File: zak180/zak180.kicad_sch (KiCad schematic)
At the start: 1 part, among them X1 25.175 MHz

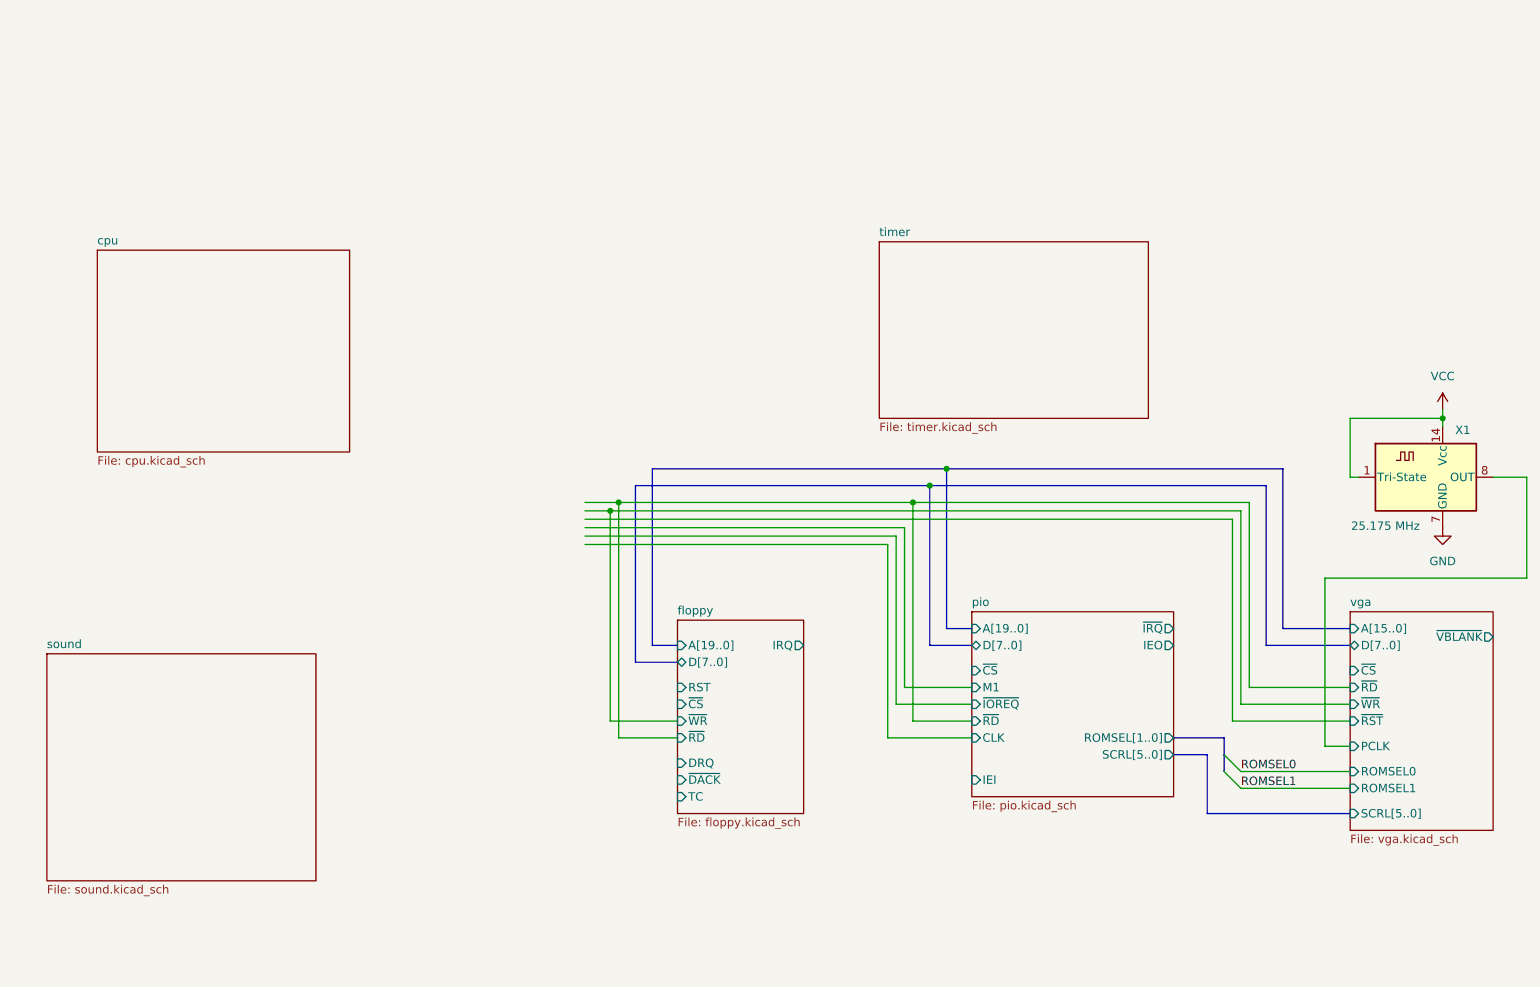
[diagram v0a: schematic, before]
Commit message: HW: Further work on schematic
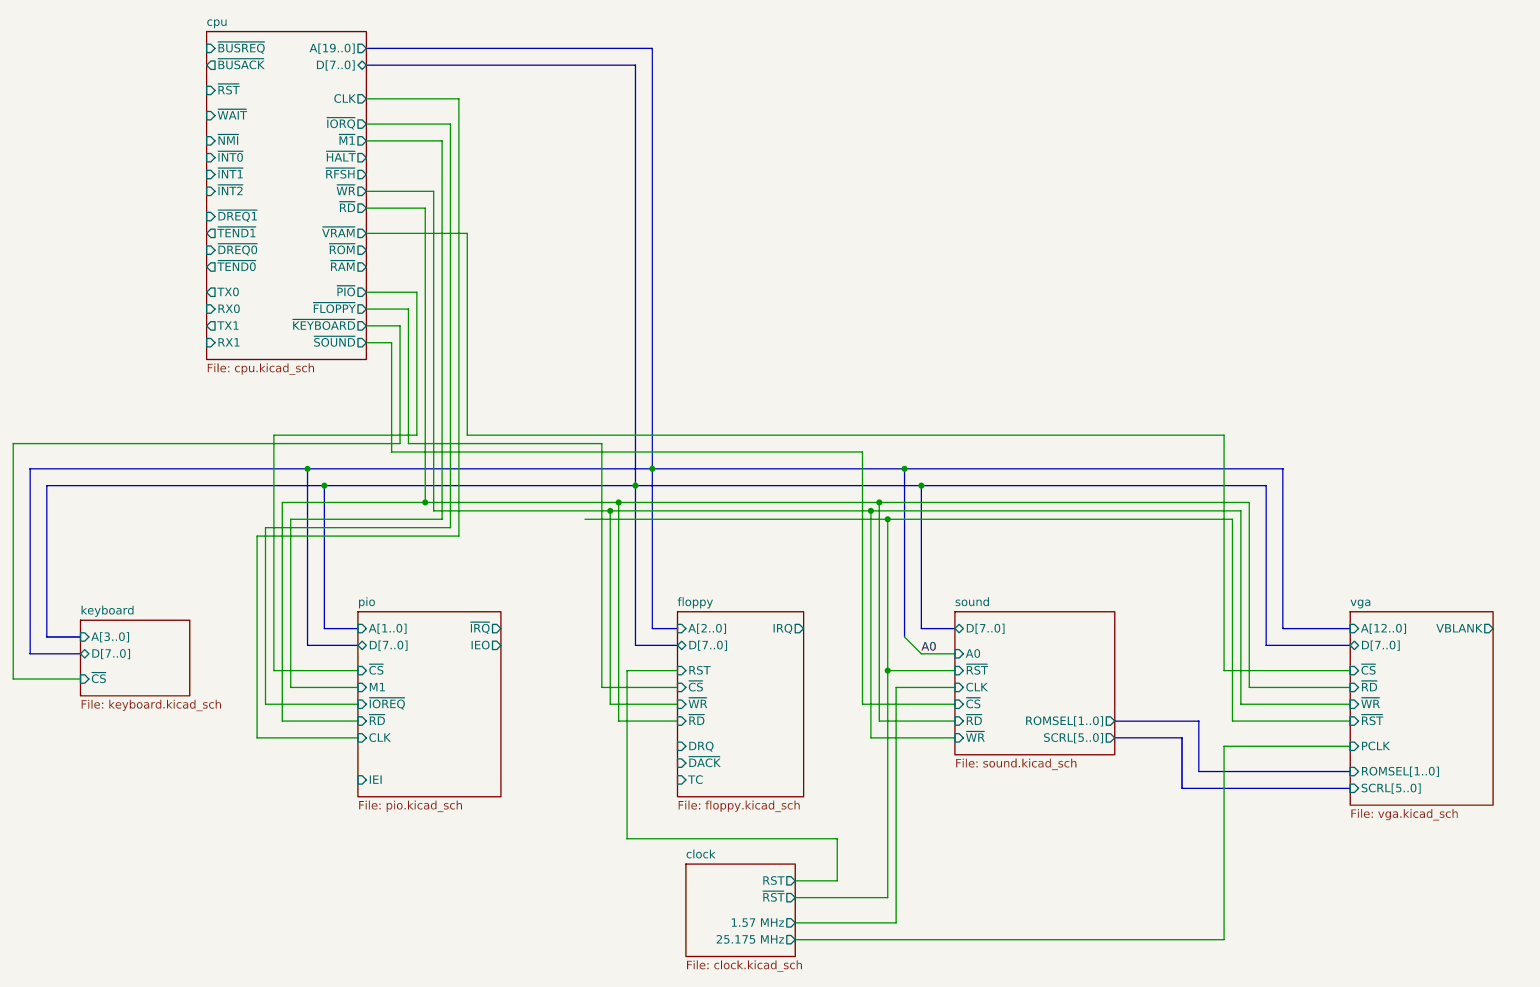
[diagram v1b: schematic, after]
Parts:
- removed X1: 25.175 MHz, Oscillator:Oscillator_DIP-14, symbol Oscillator:ACO-xxxMHz-A
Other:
- removed sheet timer
- added sheet clock (clock.kicad_sch)
- added sheet keyboard (keyboard.kicad_sch)
- sheet cpu ports: added A[19..0], CLK, D[7..0], RX0, RX1, TX0, TX1, ~{BUSACK}, ~{BUSREQ}, ~{DREQ0}, ~{DREQ1}, ~{FLOPPY}, ~{HALT}, ~{INT0}, ~{INT1}, ~{INT2}, ~{IORQ}, ~{KEYBOARD}, ~{M1}, ~{NMI}, ~{PIO}, ~{RAM}, ~{RD}, ~{RFSH}, ~{ROM}, ~{RST}, ~{SOUND}, ~{TEND0}, ~{TEND1}, ~{VRAM}, ~{WAIT}, ~{WR}; removed none
- sheet floppy ports: added A[2..0]; removed A[19..0]
- sheet pio ports: added A[1..0]; removed A[19..0], ROMSEL[1..0], SCRL[5..0]
- sheet sound ports: added A0, CLK, D[7..0], ROMSEL[1..0], SCRL[5..0], ~{CS}, ~{RD}, ~{RST}, ~{WR}; removed none
- sheet vga ports: added A[12..0], ROMSEL[1..0], VBLANK; removed A[15..0], ROMSEL0, ROMSEL1, ~{VBLANK}
